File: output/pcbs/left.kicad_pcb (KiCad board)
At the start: 2 copper layers, 127.7 x 136.5 mm, 89 parts

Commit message: add switchplate
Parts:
- removed MCU1: xiao-ble, XIAO-BLE
- moved D12 2.00 mm to (64.6, -32.4)
- moved S12 2.00 mm to (65.9, -37.2)
- moved D6 2.00 mm to (25.4, -25.3)
- moved D9 2.00 mm to (45.9, -32.2)
- moved S9 2.00 mm to (47.2, -37.0)
- moved S15 2.00 mm to (81.7, -26.8)
- moved S18 2.00 mm to (99.1, -22.1)
- moved S6 2.00 mm to (26.7, -30.1)
- moved D18 2.00 mm to (97.8, -17.3)
- moved D15 2.00 mm to (80.4, -21.9)
- moved D3 2.00 mm to (8.02, -29.9)
- moved S3 2.00 mm to (9.32, -34.8)
- moved D28 1.93 mm to (318.7, -25.3)
- moved D31 1.93 mm to (298.2, -32.2)
- moved D34 1.93 mm to (279.5, -32.4)
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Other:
- board size 127.7 x 136.5 mm -> 145 x 139.4 mm

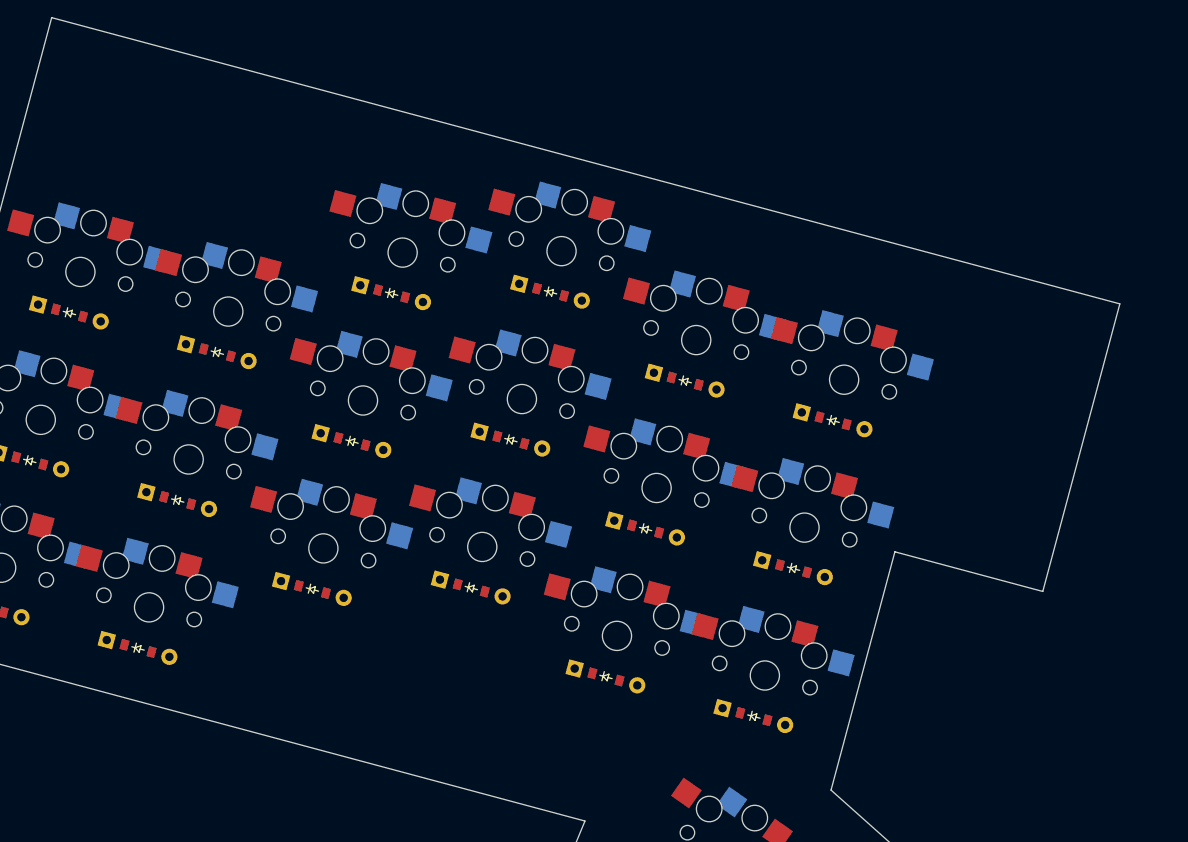
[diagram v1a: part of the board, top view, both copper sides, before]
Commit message: minimize portrusion around uhhhhhhh the uhhhhhhh xio ble
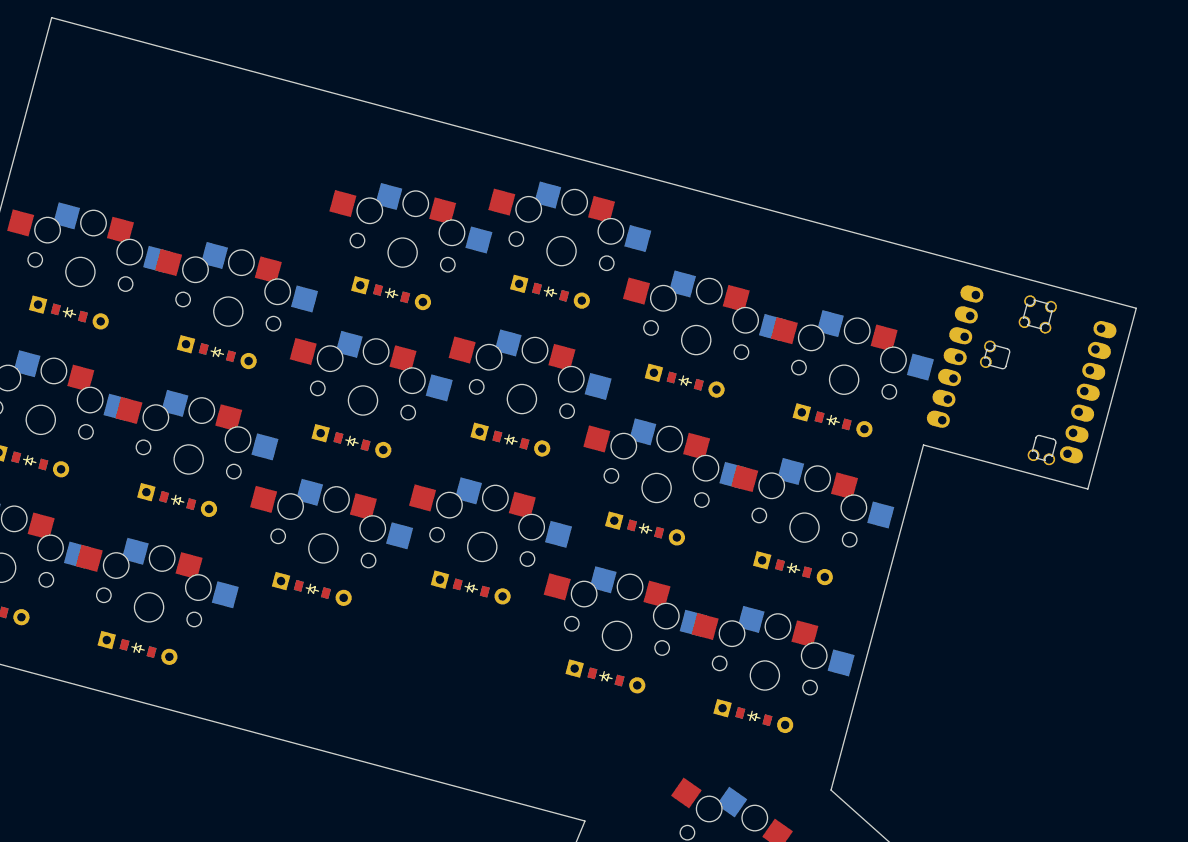
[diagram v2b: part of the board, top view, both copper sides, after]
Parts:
- added MCU1: xiao-ble, XIAO-BLE, F.Cu at (120.0, -22.7)
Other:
- board size 145 x 139.4 mm -> 146.9 x 139.4 mm
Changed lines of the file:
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@@
 (net 43 "mirror_right_bottom")
 (net 44 "mirror_right_top")
+(net 45 "P0")
+(net 46 "P1")
+(net 47 "P2")
+(net 48 "P3")
+(net 49 "P4")
+(net 50 "P5")
+(net 51 "P6")
+(net 52 "RAW5V")
+(net 53 "GND")
+(net 54 "RAW3V3")
+(net 55 "P10")
+(net 56 "P9")
+(net 57 "P8")
+(net 58 "P7")
+(net 59 "SWCLK")
+(net 60 "SWDIO")
+(net 61 "RST")
+(net 62 "BAT_POS")
+(net 63 "BAT_NEG")
+(net 64 "NFC0")
+(net 65 "NFC1")
   (net_class Default "This is the default net class."
     (clearance 0.2)
@@
 (add_net "mirror_right_bottom")
 (add_net "mirror_right_top")
+(add_net "P0")
+(add_net "P1")
+(add_net "P2")
+(add_net "P3")
+(add_net "P4")
+(add_net "P5")
+(add_net "P6")
+(add_net "RAW5V")
+(add_net "GND")
+(add_net "RAW3V3")
+(add_net "P10")
+(add_net "P9")
+(add_net "P8")
+(add_net "P7")
+(add_net "SWCLK")
+(add_net "SWDIO")
+(add_net "RST")
+(add_net "BAT_POS")
+(add_net "BAT_NEG")
+(add_net "NFC0")
+(add_net "NFC1")
   )
       (module PG1350 (layer F.Cu)
@@
         (pad 2 thru_hole circle (at 3.81 0 35) (size 1.905 1.905) (drill 0.9906) (layers *.Cu *.Mask) (net 44 "mirror_right_top"))
     )
-  (gr_line (start 122.4509257 2.7876174000000002) (end 131.5095922 -31.0197867) (angle 90) (layer Edge.Cuts) (width 0.15))
-(gr_line (start 131.5095922 -31.0197867) (end 5.939234800000001 -64.6662625) (angle 90) (layer Edge.Cuts) (width 0.15))
+    (module XIAO-BLE (layer F.Cu)
+      (at 119.9692503 -22.723974000000002 -15)
+      (fp_text reference "MCU1" (at -19.3989 -11.28268) (layer F.SilkS) hide
+        (effects (font (size 0.889 0.889) (thickness 0.1016)))
+      )
+      (fp_text value "xiao-ble" (at -19.8434 -0.29718) (layer F.SilkS) hide
+        (effects (font (size 0.6096 0.6096) (thickness 0.0762)))
+      )
+      (fp_rect (start -8.89 10.5) (end 8.89 -10.5) (layer Dwgs.User) (width 0.12) (fill none))
+      (fp_rect (start -3.507811 -8.182813) (end -5.285811 -10.849813) (layer Dwgs.User) (width 0.12) (fill none))
+      (fp_rect (start 3.350197 -6.785813) (end 5.128197 -4.118813) (layer Dwgs.User) (width 0.12) (fill none))
+      (fp_rect (start -5.285811 -6.785813) (end -3.507811 -4.118813) (layer Dwgs.User) (width 0.12) (fill none))
+      (fp_rect (start 3.350197 -10.849813) (end 5.128197 -8.182813) (layer Dwgs.User) (width 0.12) (fill none))
+      (fp_line (start -0.8382 -8.826) (end 0.8382 -8.826) (layer Edge.Cuts) (width 0.12))
+      (fp_arc (start 1.2762 -8.5782) (end 1.524 -8.1402) (angle 148.9828048) (layer Edge.Cuts) (width 0.12))
+      (fp_line (start 1.524 -8.1402) (end 1.524 -6.4638) (layer Edge.Cuts) (width 0.12))
+      (fp_arc (start 1.2762 -6.0257) (end 0.8382 -5.778) (angle 148.9828048) (layer Edge.Cuts) (width 0.12))
+      (fp_line (start -0.8382 -5.778) (end 0.8382 -5.778) (layer Edge.Cuts) (width 0.12))
+      (fp_arc (start -1.2762 -6.0258) (end -1.524 -6.4638) (angle 148.9828349) (layer Edge.Cuts) (width 0.12))
+      (fp_line (start -1.524 -8.1402) (end -1.524 -6.4638) (layer Edge.Cuts) (width 0.12))
+      (fp_arc (start -1.2762 -8.5782) (end -0.8382 -8.826) (angle 148.9829267) (layer Edge.Cuts) (width 0.12))
+      (fp_line (start -4.0132 -2.476) (end -2.413 -2.476) (layer Edge.Cuts) (width 0.12))
+      (fp_arc (start -2.4130 -2.0950) (end -2.413 -2.476) (angle 90.00030077) (layer Edge.Cuts) (width 0.12))
+      (fp_line (start -2.032 -2.095) (end -2.032 -0.444) (layer Edge.Cuts) (width 0.12))
+      (fp_arc (start -2.4130 -0.4440) (end -2.032 -0.444) (angle 90.00030077) (layer Edge.Cuts) (width 0.12))
+      (fp_line (start -4.0132 -0.063) (end -2.413 -0.063) (layer Edge.Cuts) (width 0.12))
+      (fp_arc (start -4.4512 -0.3108) (end -4.699 -0.7488) (angle 148.9837357) (layer Edge.Cuts) (width 0.12))
+      (fp_line (start -4.699 -1.7902) (end -4.699 -0.7488) (layer Edge.Cuts) (width 0.12))
+      (fp_arc (start -4.4512 -2.2282) (end -4.0132 -2.476) (angle 148.9837357) (layer Edge.Cuts) (width 0.12))
+      (fp_line (start 3.929408 6.388408) (end 5.580408 6.388408) (layer Edge.Cuts) (width 0.12))
+      (fp_arc (start 5.5804 6.7694) (end 5.580408 6.388408) (angle 89.99999995) (layer Edge.Cuts) (width 0.12))
+      (fp_line (start 5.961408 6.769408) (end 5.961408 8.369608) (layer Edge.Cuts) (width 0.12))
+      (fp_arc (start 5.7137 8.8077) (end 5.275608 9.055408) (angle 148.9852872) (layer Edge.Cuts) (width 0.12))
+      (fp_line (start 4.234208 9.055408) (end 5.275608 9.055408) (layer Edge.Cuts) (width 0.12))
+      (fp_arc (start 3.7962 8.8077) (end 3.548408 8.369608) (angle 148.9843563) (layer Edge.Cuts) (width 0.12))
+      (fp_line (start 3.548408 6.769408) (end 3.548408 8.369608) (layer Edge.Cuts) (width 0.12))
+      (fp_arc (start 3.9294 6.7694) (end 3.548408 6.769392) (angle 90.00240617) (layer Edge.Cuts) (width 0.12))
+      (pad "1" thru_hole oval (at -7.62 -7.62 -15) (size 2.75 1.8) (drill 1 (offset -0.475 0)) (layers *.Cu *.Mask) (net 45 "P0"))
+      (pad "2" thru_hole oval (at -7.62 -5.08 -15) (size 2.75 1.8) (drill 1 (offset -0.475 0)) (layers *.Cu *.Mask) (net 46 "P1"))
+      (pad "3" thru_hole oval (at -7.62 -2.54 -15) (size 2.75 1.8) (drill 1 (offset -0.475 0)) (layers *.Cu *.Mask) (net 47 "P2"))
+      (pad "4" thru_hole oval (at -7.62 0 -15) (size 2.75 1.8) (drill 1 (offset -0.475 0)) (layers *.Cu *.Mask) (net 48 "P3"))
+      (pad "5" thru_hole oval (at -7.62 2.54 -15) (size 2.75 1.8) (drill 1 (offset -0.475 0)) (layers *.Cu *.Mask) (net 49 "P4"))
+      (pad "6" thru_hole oval (at -7.62 5.08 -15) (size 2.75 1.8) (drill 1 (offset -0.475 0)) (layers *.Cu *.Mask) (net 50 "P5"))
+      (pad "7" thru_hole oval (at -7.62 7.62 -15) (size 2.75 1.8) (drill 1 (offset -0.475 0)) (layers *.Cu *.Mask) (net 51 "P6"))
+      (pad "8" thru_hole oval (at 7.62 7.62 165) (size 2.75 1.8) (drill 1 (offset -0.475 0)) (layers *.Cu *.Mask) (net 58 "P7"))
+      (pad "9" thru_hole oval (at 7.62 5.08 165) (size 2.75 1.8) (drill 1 (offset -0.475 0)) (layers *.Cu *.Mask) (net 57 "P8"))
+      (pad "10" thru_hole oval (at 7.62 2.54 165) (size 2.75 1.8) (drill 1 (offset -0.475 0)) (layers *.Cu *.Mask) (net 56 "P9"))
+      (pad "11" thru_hole oval (at 7.62 0 165) (size 2.75 1.8) (drill 1 (offset -0.475 0)) (layers *.Cu *.Mask) (net 55 "P10"))
+      (pad "12" thru_hole oval (at 7.62 -2.54 165) (size 2.75 1.8) (drill 1 (offset -0.475 0)) (layers *.Cu *.Mask) (net 54 "RAW3V3"))
+      (pad "13" thru_hole oval (at 7.62 -5.08 165) (size 2.75 1.8) (drill 1 (offset -0.475 0)) (layers *.Cu *.Mask) (net 53 "GND"))
+      (pad "14" thru_hole oval (at 7.62 -7.62 165) (size 2.75 1.8) (drill 1 (offset -0.475 0)) (layers *.Cu *.Mask) (net 52 "RAW5V"))
+      (pad "15" thru_hole circle (at -1.27 -8.572 75) (size 1.397 1.397) (drill 1.016) (layers *.Cu *.Mask) (net 59 "SWCLK"))
+      (pad "16" thru_hole circle (at 1.27 -8.572 75) (size 1.397 1.397) (drill 1.016) (layers *.Cu *.Mask) (net 60 "SWDIO"))
+      (pad "17" thru_hole circle (at -1.27 -6.032 75) (size 1.397 1.397) (drill 1.016) (layers *.Cu *.Mask) (net 53 "GND"))
+      (pad "18" thru_hole circle (at 1.27 -6.032 75) (size 1.397 1.397) (drill 1.016) (layers *.Cu *.Mask) (net 61 "RST"))
+      (pad "19" thru_hole circle (at -4.445 -0.317 165) (size 1.397 1.397) (drill 1.016) (layers *.Cu *.Mask) (net 62 "BAT_POS"))
+      (pad "20" thru_hole circle (at -4.445 -2.222 165) (size 1.397 1.397) (drill 1.016) (layers *.Cu *.Mask) (net 63 "BAT_NEG"))
+      (pad "21" thru_hole circle (at 3.802408 8.801408 255) (size 1.397 1.397) (drill 1.016) (layers *.Cu *.Mask) (net 64 "NFC0"))
+      (pad "22" thru_hole circle (at 5.707408 8.801408 255) (size 1.397 1.397) (drill 1.016) (layers *.Cu *.Mask) (net 65 "NFC1"))
+    )
+  (gr_line (start 127.7474249 -9.251780299999998) (end 133.4414439 -30.5021486) (angle 90) (layer Edge.Cuts) (width 0.15))
+(gr_line (start 133.4414439 -30.5021486) (end 5.939234800000001 -64.6662625) (angle 90) (layer Edge.Cuts) (width 0.15))
 (gr_line (start 5.939234800000001 -64.6662625) (end -13.4721936 7.7781746) (angle 90) (layer Edge.Cuts) (width 0.15))
 (gr_line (start -13.4721936 7.7781746) (end 68.6315017 29.7777934) (angle 90) (layer Edge.Cuts) (width 0.15))
@@
 (gr_line (start 92.3028306 74.6899311) (end 115.245888 41.9238493) (angle 90) (layer Edge.Cuts) (width 0.15))
 (gr_line (start 115.245888 41.9238493) (end 97.5585085 26.1407236) (angle 90) (layer Edge.Cuts) (width 0.15))
-(gr_line (start 97.5585085 26.1407236) (end 105.0642608 -1.8711254) (angle 90) (layer Edge.Cuts) (width 0.15))
-(gr_line (start 105.0642608 -1.8711254) (end 122.4509257 2.7876174000000002) (angle 90) (layer Edge.Cuts) (width 0.15))
+(gr_line (start 97.5585085 26.1407236) (end 108.4289084 -14.428161199999998) (angle 90) (layer Edge.Cuts) (width 0.15))
+(gr_line (start 108.4289084 -14.428161199999998) (end 127.7474249 -9.251780299999998) (angle 90) (layer Edge.Cuts) (width 0.15))
 )
